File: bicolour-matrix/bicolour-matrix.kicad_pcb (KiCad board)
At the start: 2 copper layers, 50 parts, among them J1 Conn_01x04_Pin, U1 HT16K33A-28SOP, U2 HT16K33A-28SOP, U3 HT16K33A-28SOP, U4 HT16K33A-28SOP

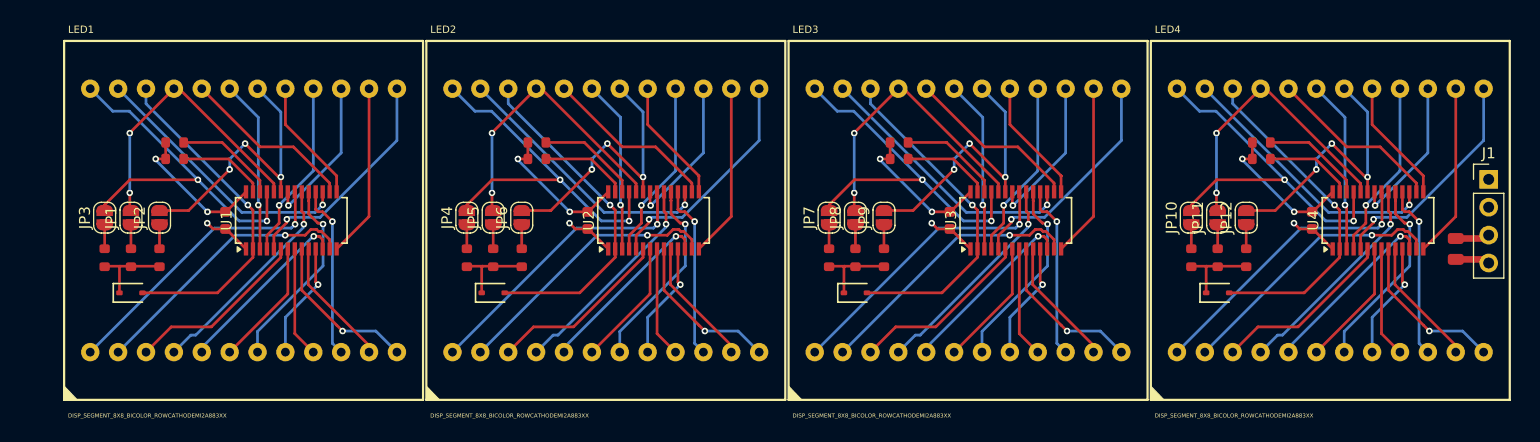
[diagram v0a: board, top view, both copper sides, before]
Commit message: feat: final revs
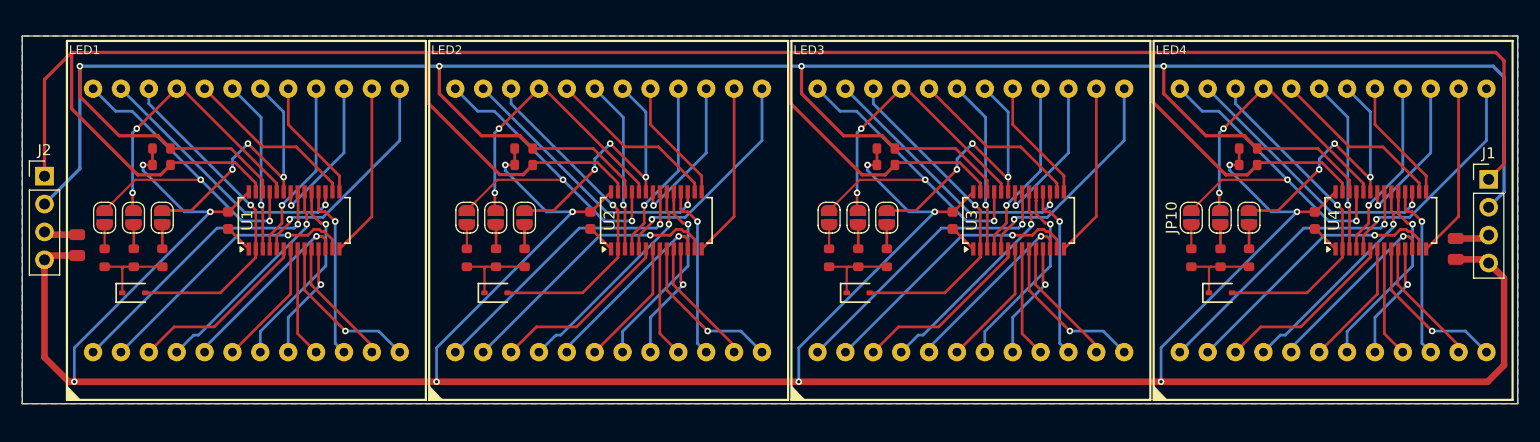
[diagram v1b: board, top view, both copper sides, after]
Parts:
- added C6: 10uF, PCM_JLCPCB:C_0805, F.Cu at (90.0, 90.0)
- added J2: Conn_01x04_Pin, Connector_PinHeader_2.54mm:PinHeader_1x04_P2.54mm_Vertical, F.Cu at (87.0, 83.8)
- moved R12 1.32 mm to (163.7, 81.2)
- moved R6 1.32 mm to (163.7, 82.8)
- moved R7 1.32 mm to (97.7, 82.8)
- moved R8 1.32 mm to (97.7, 81.2)
- moved R1 1.32 mm to (130.7, 82.8)
- moved R16 1.32 mm to (196.7, 82.8)
- moved R17 1.32 mm to (196.7, 81.2)
- moved R2 1.32 mm to (130.7, 81.2)
- moved D2 0.26 mm to (128.2, 94.4)
- moved R4 0.26 mm to (128.2, 91.2)
- moved C3 0.26 mm to (136.8, 87.8)
- moved C4 0.26 mm to (169.8, 87.8)
- moved C5 0.26 mm to (202.8, 87.8)
- moved D1 0.26 mm to (95.2, 94.4)
- moved D3 0.26 mm to (161.2, 94.4)
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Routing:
- net VDD: track 57.6 -> 301.4 mm, vias 8 -> 12
- net /Matrix 1/SDA: track 32.1 -> 260.8 mm
- net /Matrix 1/SCL: track 37.7 -> 251.4 mm, vias 0 -> 4
- net GND: track 21.1 -> 16.7 mm, vias 4 -> 0
- added copper zone on B.Cu, net GND
- added copper zone on F.Cu, net GND
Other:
- board outline added: 136.2 x 33.5 mm
